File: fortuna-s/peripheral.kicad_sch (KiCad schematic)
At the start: 15 parts, among them J1 Ext Pinout, J3 SDCard, U10 74HC74, U9 ATmega8-16P

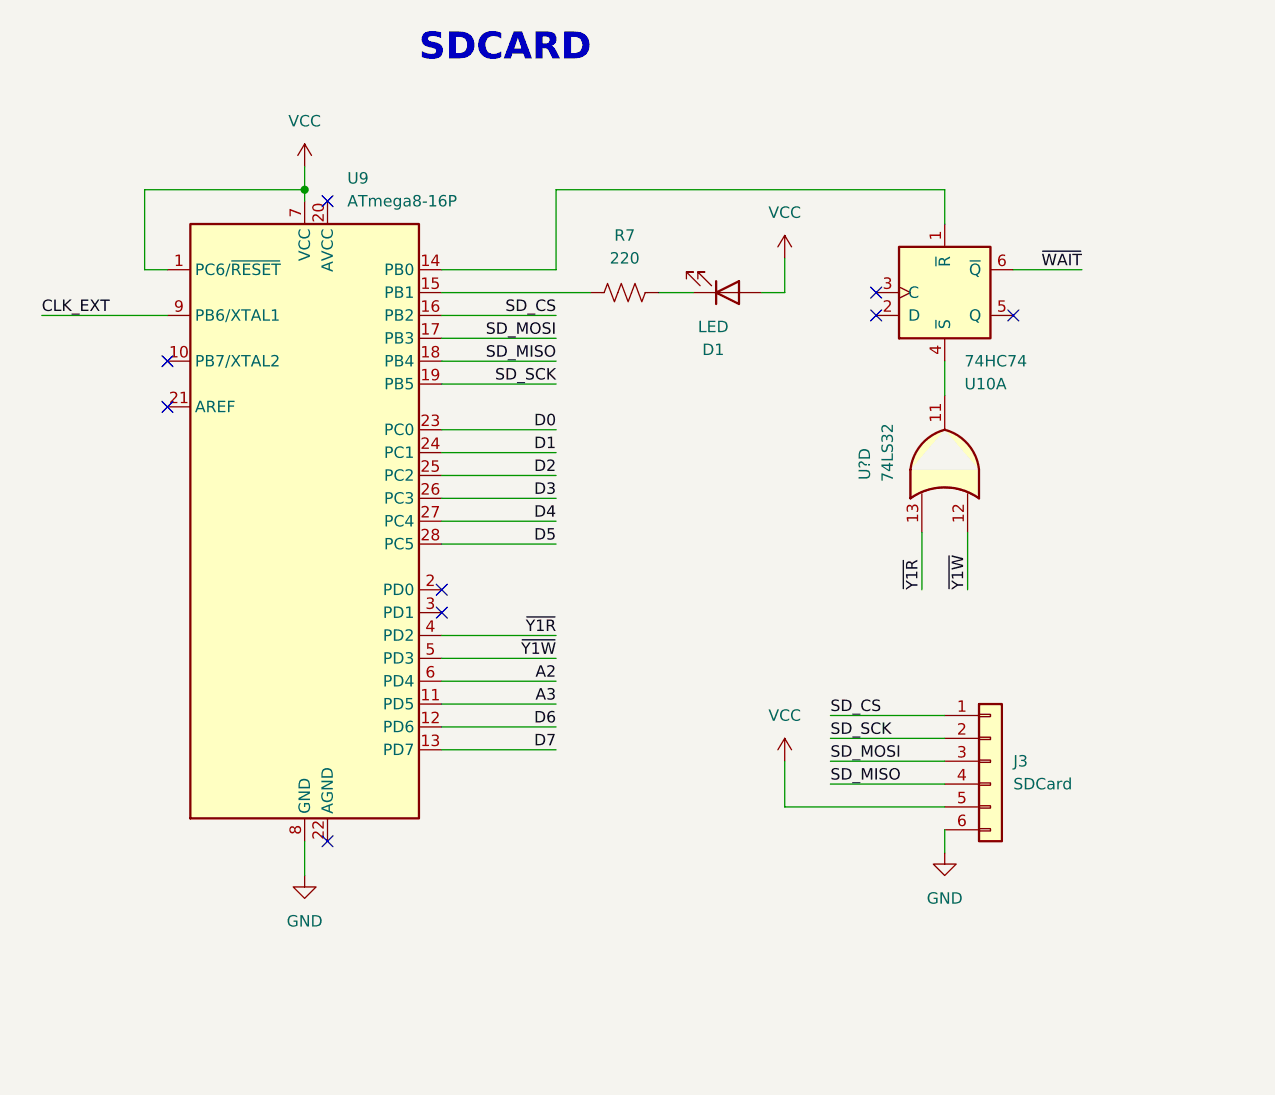
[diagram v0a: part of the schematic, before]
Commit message: .
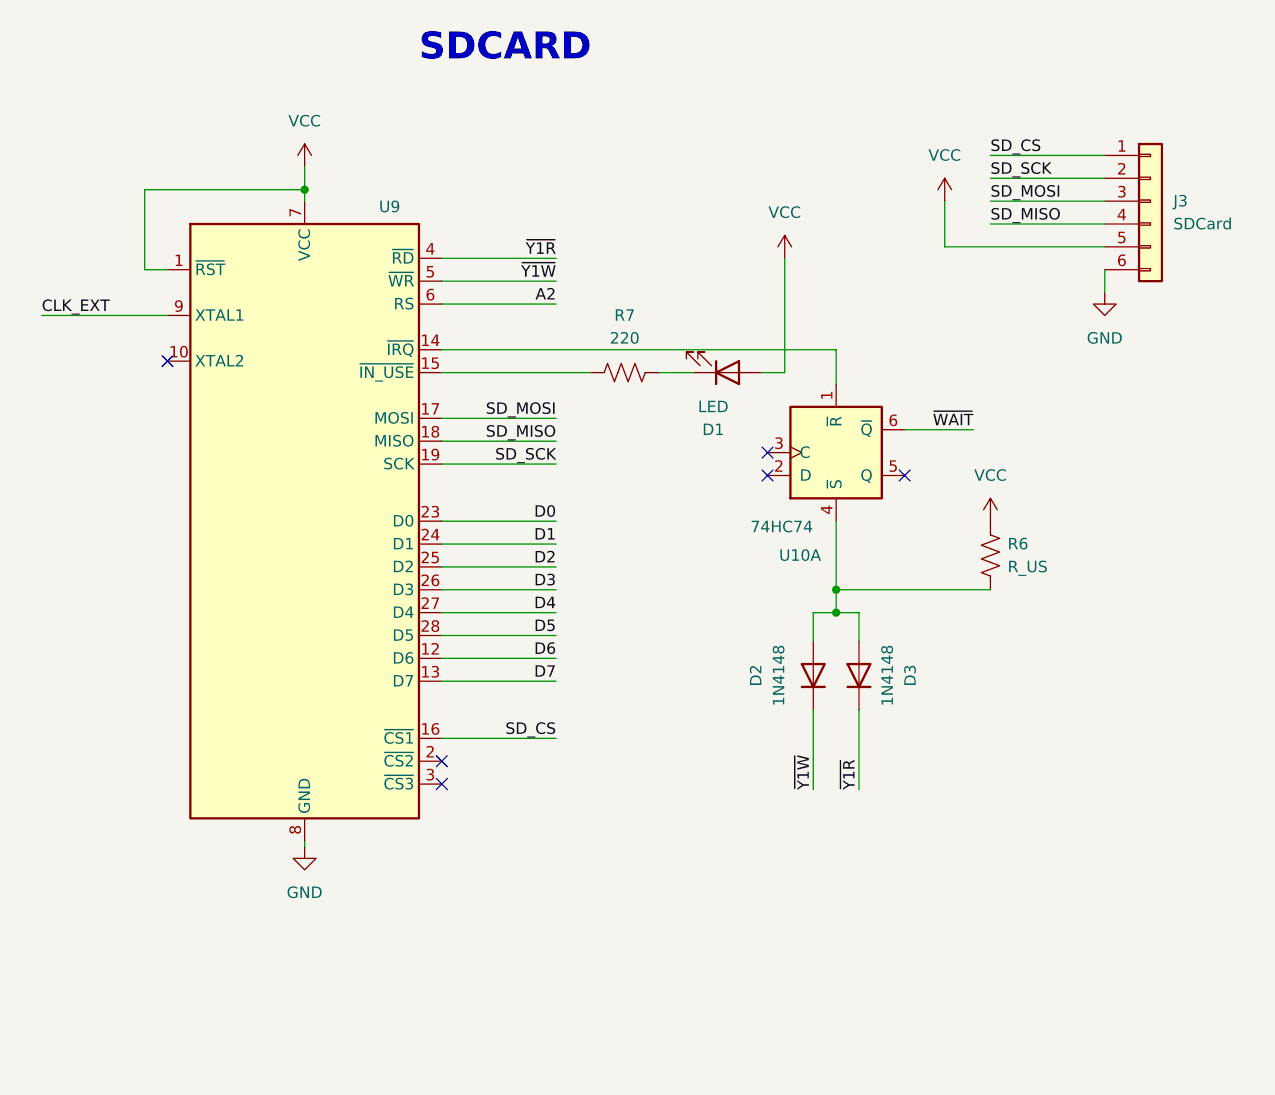
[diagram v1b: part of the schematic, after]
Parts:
- removed U9: ATmega8-16P, Package_DIP:DIP-28_W7.62mm, symbol MCU_Microchip_ATmega:ATmega8-16P
- removed U?: 74LS32, symbol 74xx:74LS32
- added D2, D3: 1N4148, Diode_THT:D_DO-35_SOD27_P7.62mm_Horizontal, symbol Diode:1N4148
- added R6: R_US, symbol Device:R_US
- added U9: ~, symbol parallel-to-spi:Parallel_to_SPI
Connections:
- net A2: now also U9.6 (RS)
- net CLK_EXT: now also U9.9 (XTAL1)
- net D0: now also U9.23 (D0)
- net D1: now also U9.24 (D1)
- net D2: now also U9.25 (D2)
- net D3: now also U9.26 (D3)
- net D4: now also U9.27 (D4)
- net D5: now also U9.28 (D5)
- net D6: now also U9.12 (D6)
- net D7: now also U9.13 (D7)
- net GND: now also U9.8 (GND)
- net SD_CS: now also U9.16 (~{CS1})
- net SD_MISO: now also U9.18 (MISO)
- net SD_MOSI: now also U9.17 (MOSI)
- net SD_SCK: now also U9.19 (SCK)
- net VCC: now also R6.1, U9.1 (~{RST}), U9.7 (VCC)
- net ~{Y1R}: now also D3.1 (K), U9.4 (~{RD})
- net ~{Y1W}: now also D2.1 (K), U9.5 (~{WR})
- net at U10.1 (~{R}): now also U9.14 (~{IRQ})
- net at R7.1: now also U9.15 (~{IN_USE})
- net at U10.4 (~{S}): now also D2.2 (A), D3.2 (A), R6.2
- no-connect marks 14 -> 11
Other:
- moved on the sheet: D1, J3, R7, U10A
